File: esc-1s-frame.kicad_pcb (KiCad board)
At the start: 4 copper layers, 26.7 x 18 mm, 21 parts, among them J1 Bat, J2 Conn_01x04_MountingPin, J4 Motor, J5 Conn_01x03_MountingPin, U1 EFM8BB51F2G-A-QFN20

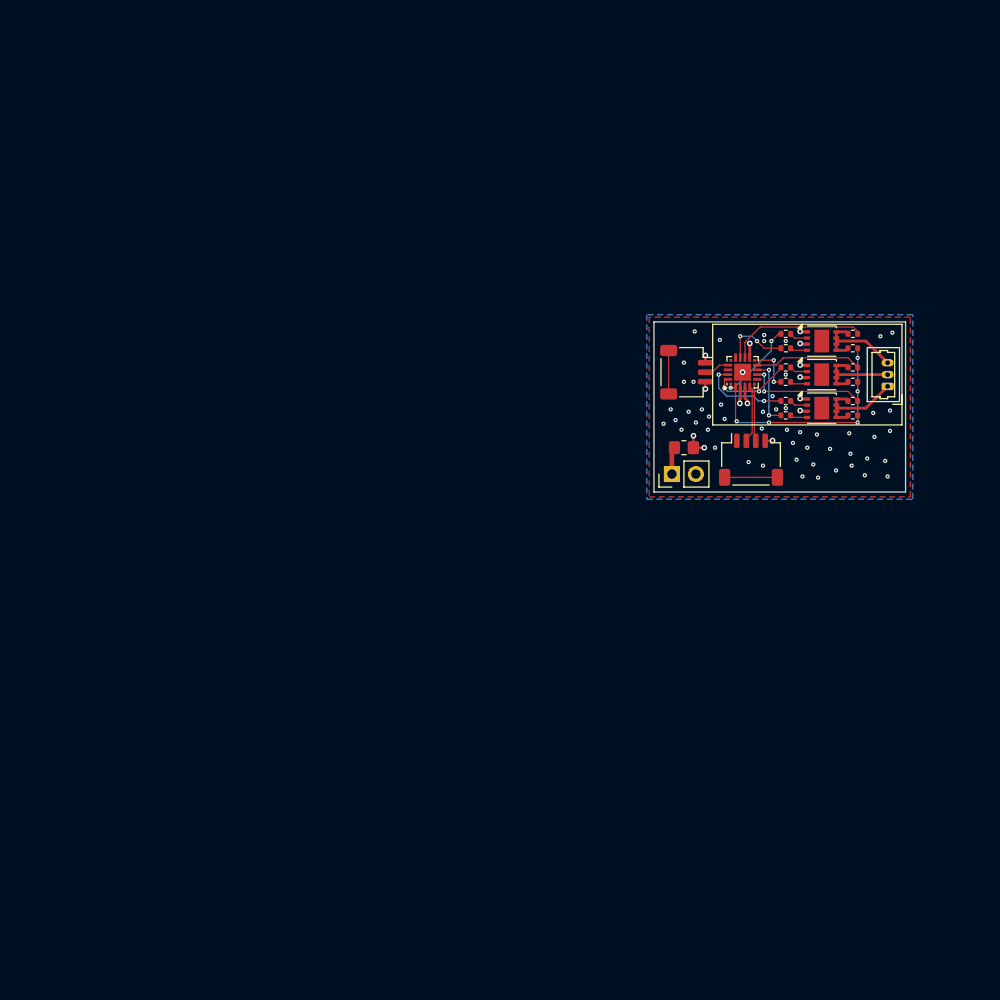
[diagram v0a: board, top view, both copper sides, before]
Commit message: full board, sent to jlcpcb
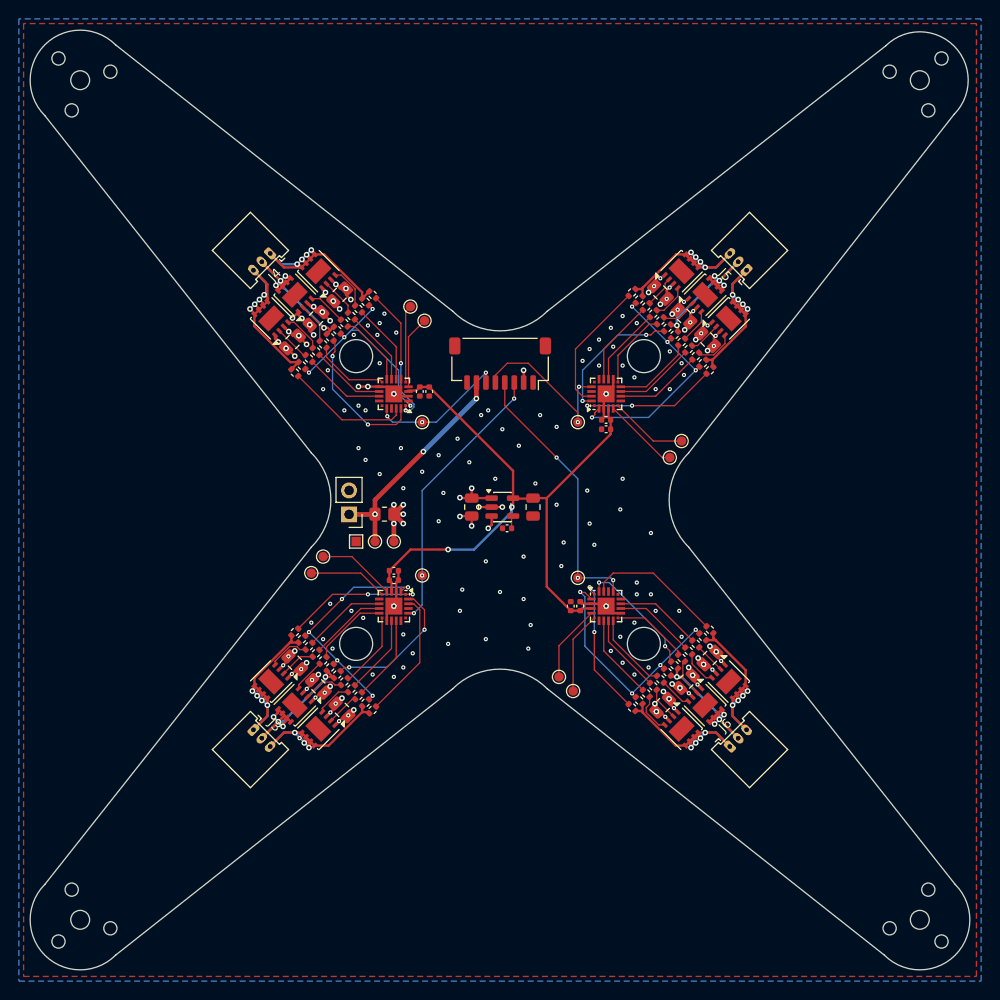
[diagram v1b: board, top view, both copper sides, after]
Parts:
- added C1: 100nF, Capacitor_SMD:C_0402_1005Metric, F.Cu at (90.8, 86.5)
- added C10: 10uF, Capacitor_SMD:C_0805_2012Metric, F.Cu at (80.0, 117.8)
- added C11: 10uF, Capacitor_SMD:C_0805_2012Metric, F.Cu at (82.5, 120.2)
- added C12: 1uF, Capacitor_SMD:C_0402_1005Metric, F.Cu at (88.0, 105.5)
- added C13: 100nF, Capacitor_SMD:C_0402_1005Metric, F.Cu at (88.0, 106.5)
- added C14: 10uF, Capacitor_SMD:C_0805_2012Metric, F.Cu at (116.2, 76.0)
- added C15: 10uF, Capacitor_SMD:C_0805_2012Metric, F.Cu at (118.8, 78.5)
- added C16: 10uF, Capacitor_SMD:C_0805_2012Metric, F.Cu at (121.2, 81.0)
- added C17: 1uF, Capacitor_SMD:C_0402_1005Metric, F.Cu at (110.5, 90.5)
- added C18: 100nF, Capacitor_SMD:C_0402_1005Metric, F.Cu at (110.5, 89.5)
- added C19: 10uF, Capacitor_SMD:C_0805_2012Metric, F.Cu at (121.5, 114.8)
- added C2: 1uF, Capacitor_SMD:C_0402_1005Metric, F.Cu at (91.8, 86.5)
- added C20: 10uF, Capacitor_SMD:C_0805_2012Metric, F.Cu at (116.5, 119.8)
- added C21: 10uF, Capacitor_SMD:C_0805_2012Metric, F.Cu at (119.0, 117.2)
- added C22: 1uF, Capacitor_SMD:C_0402_1005Metric, F.Cu at (106.8, 109.2)
- added C23: 100nF, Capacitor_SMD:C_0402_1005Metric, F.Cu at (107.8, 109.2)
- added C3: 10uF, Capacitor_SMD:C_0805_2012Metric, F.Cu at (82.2, 76.2)
- added C4: 10uF, Capacitor_SMD:C_0805_2012Metric, F.Cu at (79.8, 78.8)
- added C5: 10uF, Capacitor_SMD:C_0805_2012Metric, F.Cu at (77.2, 81.2)
- added C6: 10uF, Capacitor_SMD:C_0805_2012Metric, F.Cu at (102.8, 98.8)
- added C7: 10uF, Capacitor_SMD:C_0805_2012Metric, F.Cu at (96.2, 98.8)
- added C8: 100nF, Capacitor_SMD:C_0402_1005Metric, F.Cu at (100.0, 101.0)
- added C9: 10uF, Capacitor_SMD:C_0805_2012Metric, F.Cu at (77.5, 115.2)
- added J3: M4, Connector_Molex:Molex_PicoBlade_53048-0310_1x03_P1.25mm_Horizontal, F.Cu at (73.1, 122.4)
- added J6: M3, Connector_Molex:Molex_PicoBlade_53048-0310_1x03_P1.25mm_Horizontal, F.Cu at (123.6, 124.1)
- added R14: 100k, Resistor_SMD:R_0402_1005Metric, F.Cu at (85.8, 120.2)
- added R15: 33R, Resistor_SMD:R_0402_1005Metric, F.Cu at (84.2, 118.8)
- added R16: 33R, Resistor_SMD:R_0402_1005Metric, F.Cu at (83.5, 118.0)
- added R17: 10k, Resistor_SMD:R_0402_1005Metric, F.Cu at (85.0, 119.5)
- added R18: 100k, Resistor_SMD:R_0402_1005Metric, F.Cu at (82.0, 116.5)
- added R19: 33R, Resistor_SMD:R_0402_1005Metric, F.Cu at (82.8, 117.2)
- added R20: 33R, Resistor_SMD:R_0402_1005Metric, F.Cu at (80.5, 115.0)
- added R21: 10k, Resistor_SMD:R_0402_1005Metric, F.Cu at (81.2, 115.8)
- added R22: 100k, Resistor_SMD:R_0402_1005Metric, F.Cu at (77.5, 112.0)
- added R23: 33R, Resistor_SMD:R_0402_1005Metric, F.Cu at (79.8, 114.2)
- added R24: 33R, Resistor_SMD:R_0402_1005Metric, F.Cu at (79.0, 113.5)
- added R25: 10k, Resistor_SMD:R_0402_1005Metric, F.Cu at (78.2, 112.8)
- added R26: 100k, Resistor_SMD:R_0402_1005Metric, F.Cu at (113.2, 76.0)
- added R27: 33R, Resistor_SMD:R_0402_1005Metric, F.Cu at (114.8, 77.5)
- added R28: 33R, Resistor_SMD:R_0402_1005Metric, F.Cu at (115.5, 78.2)
- added R29: 10k, Resistor_SMD:R_0402_1005Metric, F.Cu at (114.0, 76.8)
- added R30: 100k, Resistor_SMD:R_0402_1005Metric, F.Cu at (117.0, 79.8)
- added R31: 33R, Resistor_SMD:R_0402_1005Metric, F.Cu at (116.2, 79.0)
- added R32: 33R, Resistor_SMD:R_0402_1005Metric, F.Cu at (118.5, 81.2)
- added R33: 10k, Resistor_SMD:R_0402_1005Metric, F.Cu at (117.8, 80.5)
- added R34: 100k, Resistor_SMD:R_0402_1005Metric, F.Cu at (121.5, 84.2)
- added R35: 33R, Resistor_SMD:R_0402_1005Metric, F.Cu at (119.2, 82.0)
- added R36: 33R, Resistor_SMD:R_0402_1005Metric, F.Cu at (120.0, 82.8)
- added R37: 10k, Resistor_SMD:R_0402_1005Metric, F.Cu at (120.8, 83.5)
- added R38: 100k, Resistor_SMD:R_0402_1005Metric, F.Cu at (121.5, 111.8)
- added R39: 33R, Resistor_SMD:R_0402_1005Metric, F.Cu at (120.0, 113.2)
- added R40: 33R, Resistor_SMD:R_0402_1005Metric, F.Cu at (119.2, 114.0)
- added R41: 10k, Resistor_SMD:R_0402_1005Metric, F.Cu at (120.8, 112.5)
- added R42: 100k, Resistor_SMD:R_0402_1005Metric, F.Cu at (117.8, 115.5)
- added R43: 33R, Resistor_SMD:R_0402_1005Metric, F.Cu at (118.5, 114.8)
- added R44: 33R, Resistor_SMD:R_0402_1005Metric, F.Cu at (116.2, 117.0)
- added R45: 10k, Resistor_SMD:R_0402_1005Metric, F.Cu at (117.0, 116.2)
- added R46: 100k, Resistor_SMD:R_0402_1005Metric, F.Cu at (113.2, 120.0)
- added R47: 33R, Resistor_SMD:R_0402_1005Metric, F.Cu at (115.5, 117.8)
- added R48: 33R, Resistor_SMD:R_0402_1005Metric, F.Cu at (114.8, 118.5)
- added R49: 10k, Resistor_SMD:R_0402_1005Metric, F.Cu at (114.0, 119.2)
- added TP1: RX, TestPoint:TestPoint_Pad_D1.0mm, F.Cu at (91.0, 89.8)
- added TP10: C2CK, TestPoint:TestPoint_Pad_D1.0mm, F.Cu at (117.2, 93.5)
- added TP11: C2D, TestPoint:TestPoint_Pad_D1.0mm, F.Cu at (118.5, 91.8)
- added TP12: RX, TestPoint:TestPoint_Pad_D1.0mm, F.Cu at (107.5, 89.8)
- added TP13: C2CK, TestPoint:TestPoint_Pad_D1.0mm, F.Cu at (105.5, 116.8)
- added TP14: C2D, TestPoint:TestPoint_Pad_D1.0mm, F.Cu at (107.0, 118.2)
- added TP15: RX, TestPoint:TestPoint_Pad_D1.0mm, F.Cu at (107.5, 106.2)
- added TP2: sense_p, TestPoint:TestPoint_Pad_D1.0mm, F.Cu at (86.0, 102.4)
- added TP3: sense_n, TestPoint:TestPoint_Pad_D1.0mm, F.Cu at (88.0, 102.4)
- added TP4: C2CK, TestPoint:TestPoint_Pad_D1.0mm, F.Cu at (91.2, 79.0)
- added TP5: C2D, TestPoint:TestPoint_Pad_D1.0mm, F.Cu at (89.8, 77.5)
- added TP6: GND, TestPoint:TestPoint_Pad_1.0x1.0mm, F.Cu at (84.0, 102.4)
- added TP7: C2CK, TestPoint:TestPoint_Pad_D1.0mm, F.Cu at (80.5, 104.0)
- added TP8: C2D, TestPoint:TestPoint_Pad_D1.0mm, F.Cu at (79.2, 105.8)
- added TP9: RX, TestPoint:TestPoint_Pad_D1.0mm, F.Cu at (91.0, 106.0)
- added U10: XR30G30D, Package_DFN_QFN:DFN-8-1EP_3x3mm_P0.65mm_EP1.55x2.4mm, F.Cu at (118.5, 73.8)
- added U11: XR30G30D, Package_DFN_QFN:DFN-8-1EP_3x3mm_P0.65mm_EP1.55x2.4mm, F.Cu at (121.0, 76.2)
- added U12: XR30G30D, Package_DFN_QFN:DFN-8-1EP_3x3mm_P0.65mm_EP1.55x2.4mm, F.Cu at (123.5, 78.8)
- added U13: EFM8BB51F2G-A-QFN20, Package_DFN_QFN:SiliconLabs_QFN-20-1EP_3x3mm_P0.5mm_EP1.8x1.8mm, F.Cu at (110.5, 86.8)
- added U14: XR30G30D, Package_DFN_QFN:DFN-8-1EP_3x3mm_P0.65mm_EP1.55x2.4mm, F.Cu at (123.5, 117.2)
- added U15: XR30G30D, Package_DFN_QFN:DFN-8-1EP_3x3mm_P0.65mm_EP1.55x2.4mm, F.Cu at (121.0, 119.8)
- added U16: XR30G30D, Package_DFN_QFN:DFN-8-1EP_3x3mm_P0.65mm_EP1.55x2.4mm, F.Cu at (118.5, 122.2)
- added U17: EFM8BB51F2G-A-QFN20, Package_DFN_QFN:SiliconLabs_QFN-20-1EP_3x3mm_P0.5mm_EP1.8x1.8mm, F.Cu at (110.5, 109.2)
- added U5: XR30G30D, Package_DFN_QFN:DFN-8-1EP_3x3mm_P0.65mm_EP1.55x2.4mm, F.Cu at (80.0, 122.2)
- added U6: SPX3819M5-L-3-3, Package_TO_SOT_SMD:SOT-23-5, F.Cu at (99.5, 98.8)
- added U7: XR30G30D, Package_DFN_QFN:DFN-8-1EP_3x3mm_P0.65mm_EP1.55x2.4mm, F.Cu at (77.5, 119.8)
- added U8: XR30G30D, Package_DFN_QFN:DFN-8-1EP_3x3mm_P0.65mm_EP1.55x2.4mm, F.Cu at (75.0, 117.2)
- added U9: EFM8BB51F2G-A-QFN20, Package_DFN_QFN:SiliconLabs_QFN-20-1EP_3x3mm_P0.5mm_EP1.8x1.8mm, F.Cu at (88.0, 109.2)
- J2: value Conn_01x04_MountingPin -> Ctrl; footprint Connector_JST:JST_SH_SM04B-SRSS-TB_1x04-1MP_P1.00mm_Horizontal -> Connector_JST:JST_SH_SM08B-SRSS-TB_1x08-1MP_P1.00mm_Horizontal
- J4: value Motor -> M1; footprint Connector_Molex:Molex_PicoBlade_53047-0310_1x03_P1.25mm_Vertical -> Connector_Molex:Molex_PicoBlade_53048-0310_1x03_P1.25mm_Horizontal
- J5: value Conn_01x03_MountingPin -> M2; footprint Connector_JST:JST_SH_SM03B-SRSS-TB_1x03-1MP_P1.00mm_Horizontal -> Connector_Molex:Molex_PicoBlade_53048-0310_1x03_P1.25mm_Horizontal
- U2, U3, U4: value ~ -> XR30G30D
- moved J4 67.0 mm to (74.9, 71.9), turned to -135 degrees
- moved R2 59.3 mm to (77.5, 84.5), turned to 135 degrees
- moved R3 58.4 mm to (78.2, 83.8), turned to -45 degrees
- moved U2 58.4 mm to (75.0, 78.8), turned to 135 degrees
- moved U3 56.5 mm to (77.5, 76.2), turned to 135 degrees
- moved R6 55.5 mm to (81.2, 80.8), turned to 135 degrees
- moved U4 55.3 mm to (80.0, 73.8), turned to 135 degrees
- moved R9 54.9 mm to (82.0, 80.0), turned to -45 degrees
- moved R13 53.0 mm to (85.0, 77.0), turned to -45 degrees
- moved R10 52.1 mm to (85.8, 76.2), turned to 135 degrees
- moved R5 50.6 mm to (79.0, 83.0), turned to 135 degrees
- moved R4 49.8 mm to (79.8, 82.2), turned to 135 degrees
- moved R8 49.1 mm to (80.5, 81.5), turned to 135 degrees
- moved R7 47.2 mm to (82.8, 79.2), turned to 135 degrees
- moved R12 46.9 mm to (83.5, 78.5), turned to 135 degrees
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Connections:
- net /A renamed /motor1_A
- net /B renamed /motor1_B
- net /C renamed /motor1_C
- net /Vn renamed /esc1_Vn
- J2 pad 1: VDD -> /telem
- J2 pad 2: /C2CK -> VDD
- J2 pad 3: /C2D -> /esc4_rx
- J2 pad 4: -BATT -> /esc3_rx
- J5 pad 1: VDD -> /motor2_C
- J5 pad 2: Net-(J5-Pin_2) -> /motor2_B
- J5 pad 3: -BATT -> /motor2_A
- R10 pad 1: /Cc -> /esc1_Cm
- R11 pad 1: /Cp -> /esc1_Cp
- R12 pad 1: /Cm -> /esc1_Cc
- R2 pad 1: /Ac -> /esc1_Am
- R4 pad 1: /Ap -> /esc1_Ap
- R5 pad 1: /Am -> /esc1_Ac
- R6 pad 1: /Bc -> /esc1_Bm
- R7 pad 1: /Bp -> /esc1_Bp
- R8 pad 1: /Bm -> /esc1_Bc
- U1 pad 1: /Am -> /esc1_Cm
- U1 pad 10: /Bc -> /esc1_Bp
- U1 pad 11: /Bp -> /esc1_Bc
- U1 pad 13: /Ac -> /esc1_Ap
- U1 pad 14: /Ap -> /esc1_Ac
- U1 pad 17: Net-(J5-Pin_2) -> /esc1_rx
- U1 pad 19: /Cm -> /esc1_Am
- U1 pad 20: /Bm -> /esc1_Bm
- U1 pad 4: VDD -> +3V3
- U1 pad 5: /C2CK -> /esc1_C2CK
- U1 pad 6: /C2D -> /esc1_C2D
- U1 pad 8: /Cc -> /esc1_Cp
- U1 pad 9: /Cp -> /esc1_Cc
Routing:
- net +3V3: track 0.00 -> 68.5 mm, vias 0 -> 2
- net -BATT: track 7.12 -> 54.7 mm, vias 28 -> 115
- net VDD: track 7.38 -> 51.9 mm, vias 39 -> 65
- net /esc4_rx: track 0.00 -> 29.4 mm, vias 0 -> 3
- net /esc3_rx: track 0.00 -> 29.0 mm, vias 0 -> 3
- net /esc3_Vn: track 0.00 -> 25.7 mm, vias 0 -> 4
- net /esc2_Vn: track 0.00 -> 25.5 mm, vias 0 -> 4
- net /esc4_Vn: track 0.00 -> 24.6 mm, vias 0 -> 5
- net +BATT: track 2.91 -> 26.8 mm, vias 0 -> 3
- net /motor4_A: track 0.00 -> 21.4 mm, vias 0 -> 4
- net /motor3_A: track 0.00 -> 21.4 mm, vias 0 -> 4
- net /motor4_B: track 0.00 -> 21.3 mm, vias 0 -> 4
- net /motor4_C: track 0.00 -> 21.2 mm, vias 0 -> 4
- net /motor3_C: track 0.00 -> 20.9 mm, vias 0 -> 4
- net /motor2_A: track 0.00 -> 20.8 mm, vias 0 -> 4
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- added copper zone on F.Cu, net -BATT
- added copper zone on B.Cu, net VDD
- removed copper zone on B.Cu, net -BATT
- removed copper zone on F.Cu, net VDD
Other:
- board size 26.7 x 18 mm -> 99.6 x 99.6 mm
